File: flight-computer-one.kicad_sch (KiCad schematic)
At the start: 6 parts, among them J1 LEFT_BANK, J2 RIGHT_BANK

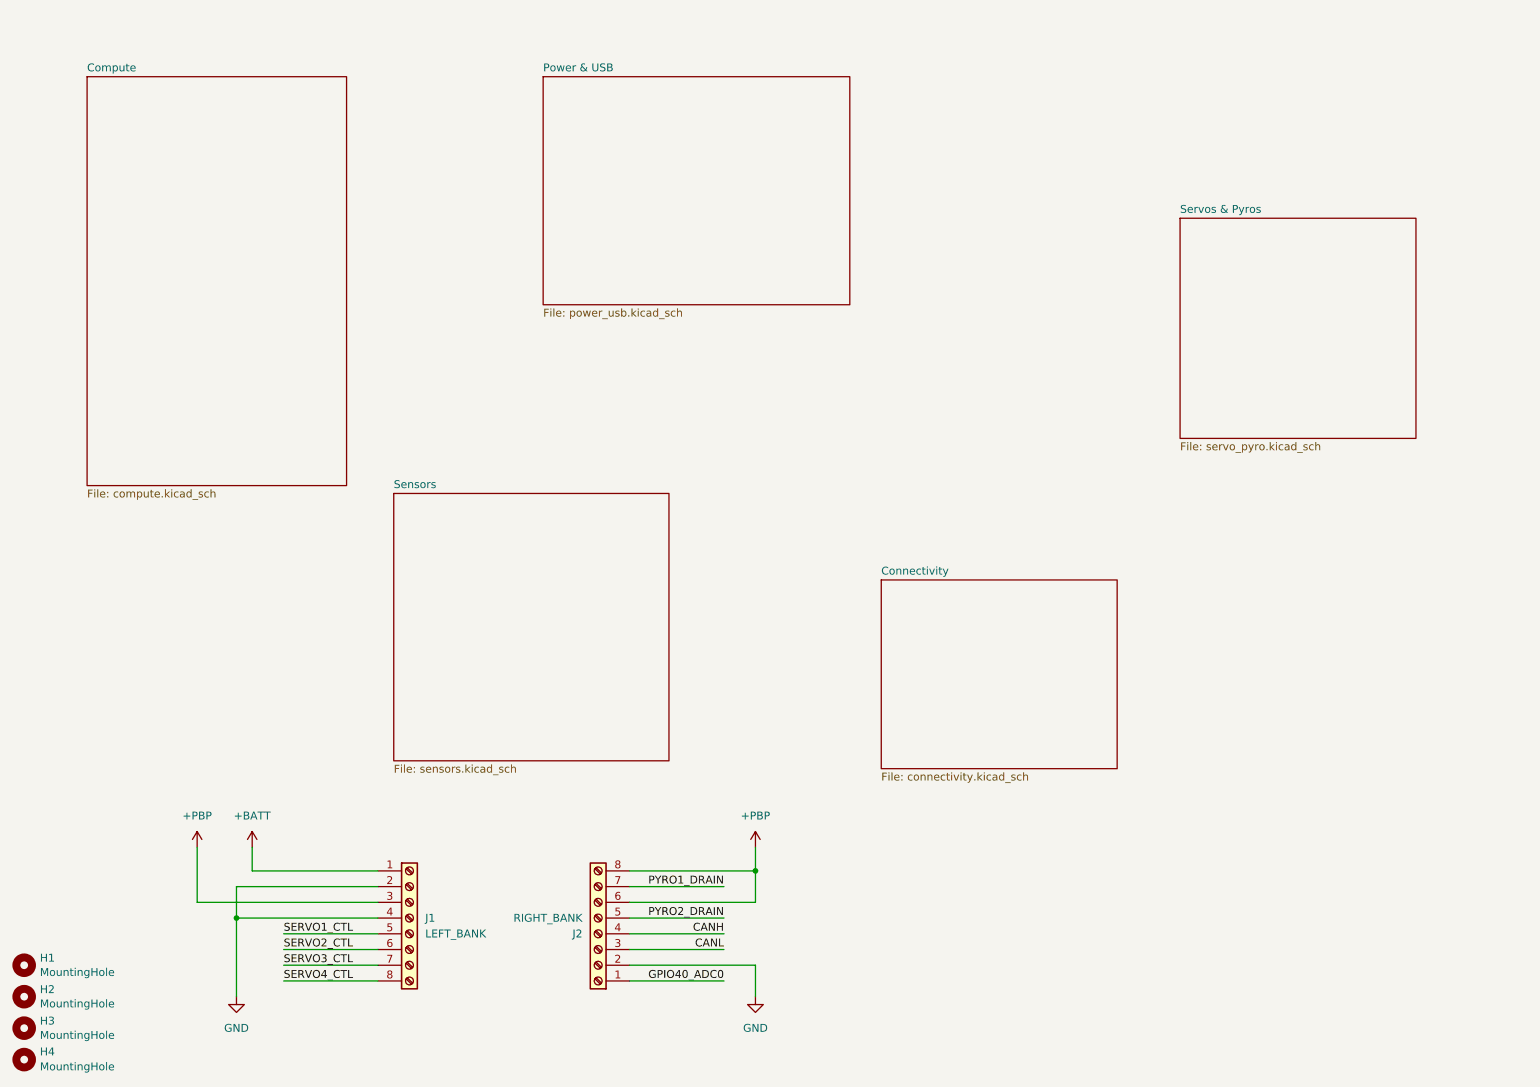
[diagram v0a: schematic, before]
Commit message: schematic tentatively finished
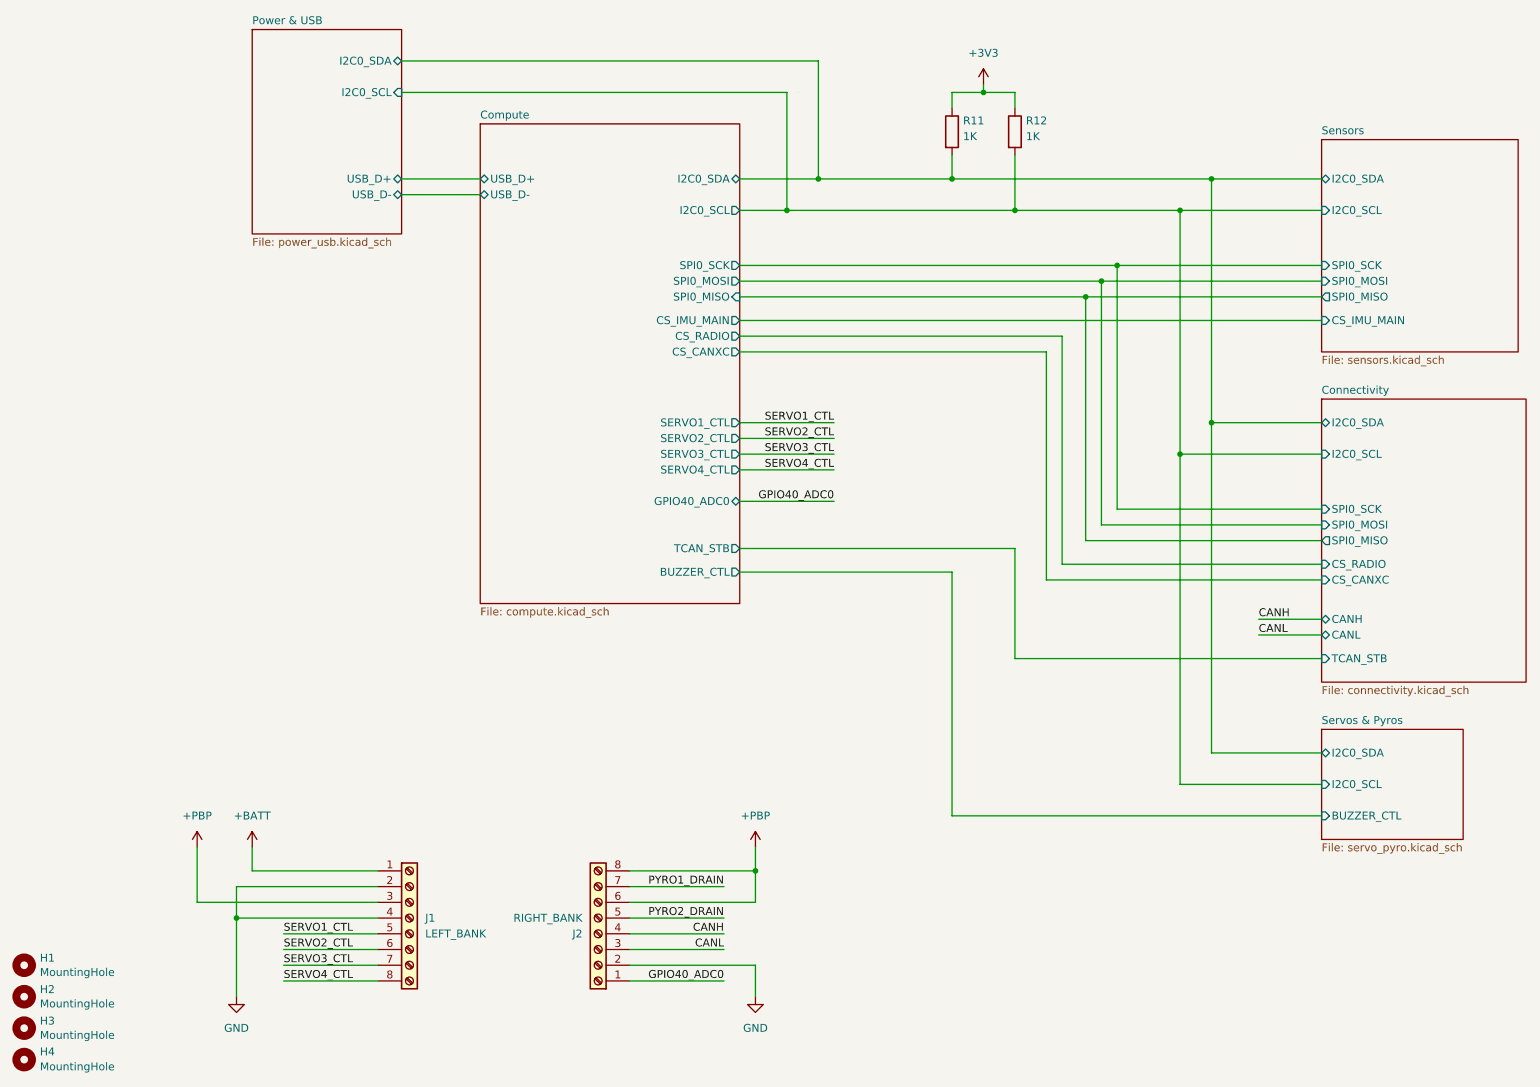
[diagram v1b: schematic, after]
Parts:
- added R11, R12: 1K, Resistor_SMD:R_0603_1608Metric, symbol Device:R
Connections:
- new net +3V3: R11.1, R12.1
- new net Compute/I2C0_SCL: R12.2
- new net Compute/I2C0_SDA: R11.2
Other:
- sheet Compute ports: added BUZZER_CTL, CS_CANXC, CS_IMU_MAIN, CS_RADIO, GPIO40_ADC0, I2C0_SCL, I2C0_SDA, SERVO1_CTL, SERVO2_CTL, SERVO3_CTL, SERVO4_CTL, SPI0_MISO, SPI0_MOSI, SPI0_SCK, TCAN_STB, USB_D+, USB_D-; removed none
- sheet Connectivity ports: added CANH, CANL, CS_CANXC, CS_RADIO, I2C0_SCL, I2C0_SDA, SPI0_MISO, SPI0_MOSI, SPI0_SCK, TCAN_STB; removed none
- sheet Power & USB ports: added I2C0_SCL, I2C0_SDA, USB_D+, USB_D-; removed none
- sheet Sensors ports: added CS_IMU_MAIN, I2C0_SCL, I2C0_SDA, SPI0_MISO, SPI0_MOSI, SPI0_SCK; removed none
- sheet Servos & Pyros ports: added BUZZER_CTL, I2C0_SCL, I2C0_SDA; removed none

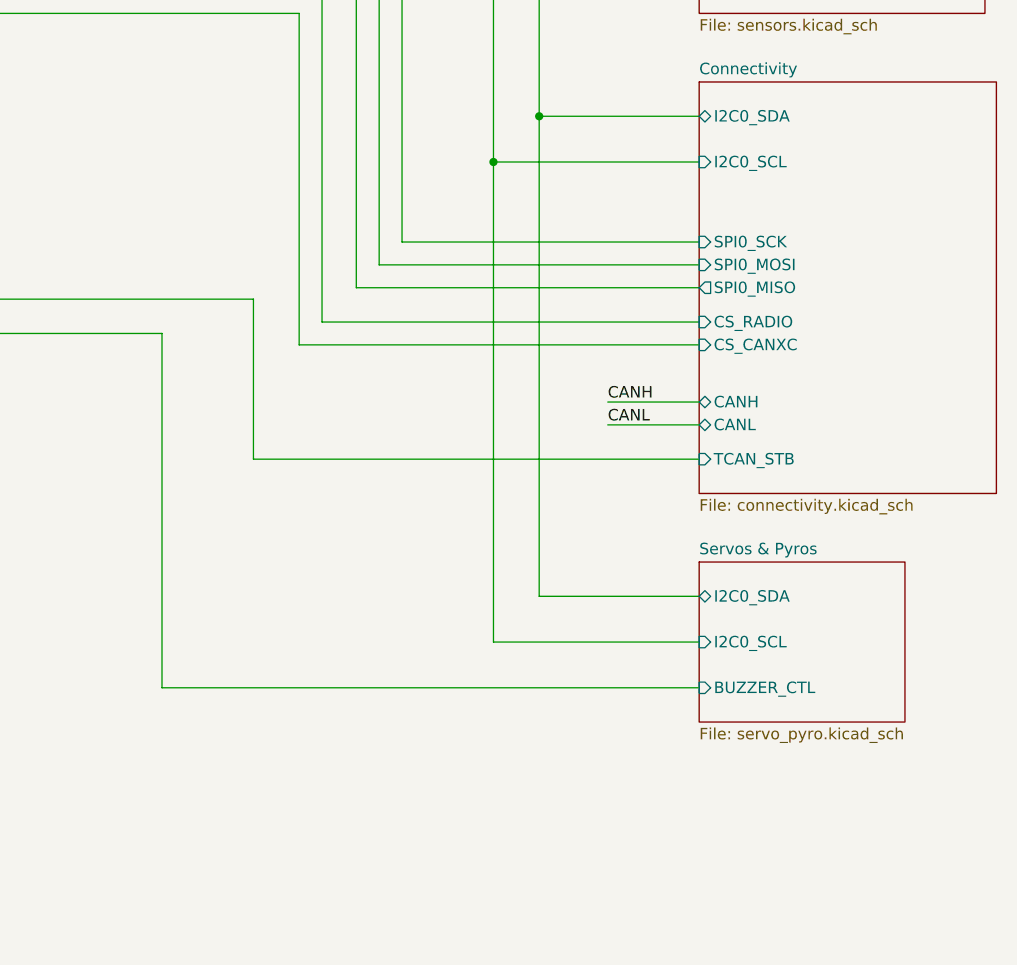
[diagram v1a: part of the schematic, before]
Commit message: preliminary change to SAME51
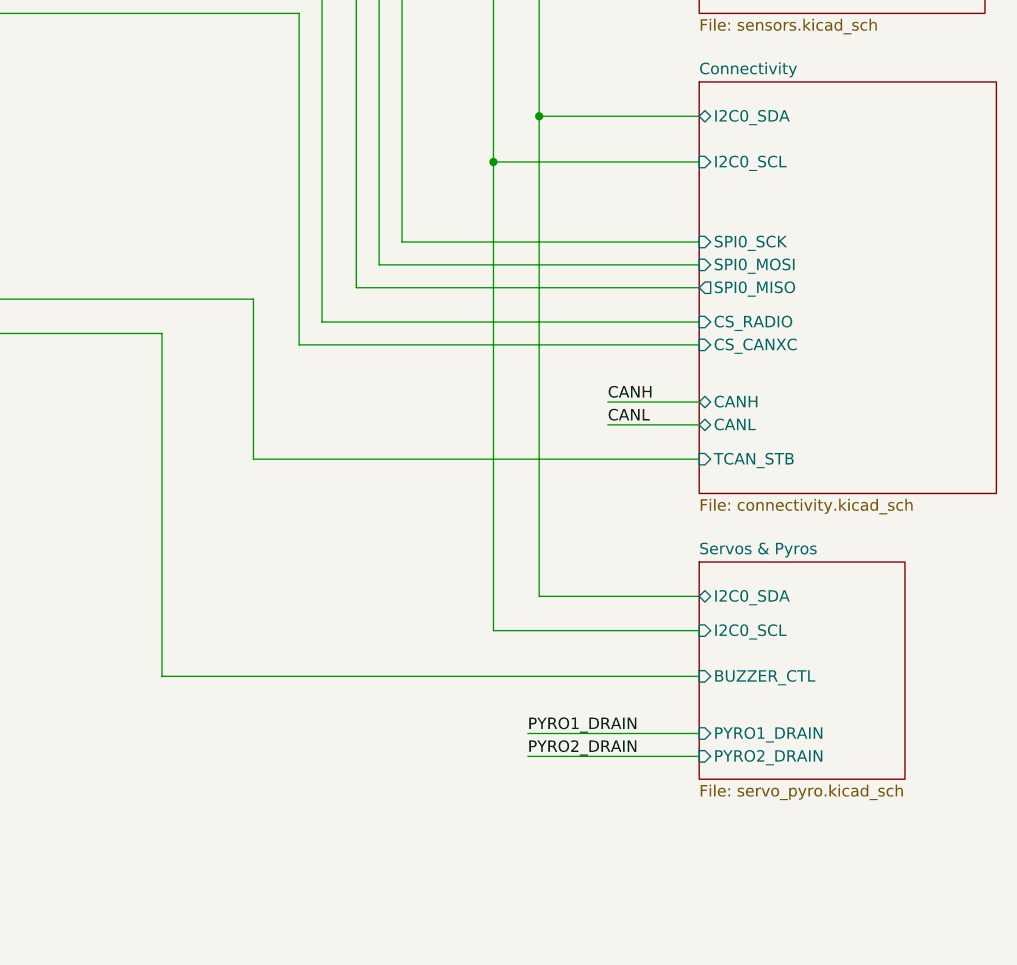
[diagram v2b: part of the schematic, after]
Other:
- sheet Servos & Pyros ports: added PYRO1_DRAIN, PYRO2_DRAIN; removed none
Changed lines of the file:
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@@
 	(wire
 		(pts
-			(xy 173.99 149.86) (xy 233.68 149.86)
+			(xy 173.99 148.59) (xy 233.68 148.59)
 		)
 		(stroke
@@
 	(wire
 		(pts
+			(xy 121.92 166.37) (xy 137.16 166.37)
+		)
+		(stroke
+			(width 0)
+			(type default)
+		)
+	)
+	(wire
+		(pts
 			(xy 184.15 43.18) (xy 184.15 52.07)
 		)
@@
 	(wire
 		(pts
+			(xy 214.63 157.48) (xy 233.68 157.48)
+		)
+		(stroke
+			(width 0)
+			(type default)
+		)
+	)
+	(wire
+		(pts
+			(xy 214.63 154.94) (xy 233.68 154.94)
+		)
+		(stroke
+			(width 0)
+			(type default)
+		)
+	)
+	(wire
+		(pts
 			(xy 223.52 118.11) (xy 233.68 118.11)
 		)
@@
 	(wire
 		(pts
-			(xy 210.82 91.44) (xy 210.82 144.78)
+			(xy 210.82 91.44) (xy 210.82 143.51)
 		)
 		(stroke
@@
 	(wire
 		(pts
-			(xy 121.92 166.37) (xy 137.16 166.37)
-		)
-		(stroke
-			(width 0)
-			(type default)
-		)
-	)
-	(wire
-		(pts
 			(xy 139.7 93.98) (xy 154.94 93.98)
 		)
@@
 	(wire
 		(pts
+			(xy 121.92 161.29) (xy 137.16 161.29)
+		)
+		(stroke
+			(width 0)
+			(type default)
+		)
+	)
+	(wire
+		(pts
 			(xy 85.09 49.53) (xy 97.79 49.53)
 		)
@@
 	(wire
 		(pts
-			(xy 121.92 161.29) (xy 137.16 161.29)
-		)
-		(stroke
-			(width 0)
-			(type default)
-		)
-	)
-	(wire
-		(pts
 			(xy 179.07 31.75) (xy 179.07 33.02)
 		)
@@
 	(wire
 		(pts
-			(xy 210.82 144.78) (xy 233.68 144.78)
+			(xy 210.82 143.51) (xy 233.68 143.51)
 		)
 		(stroke
@@
 	(wire
 		(pts
-			(xy 173.99 110.49) (xy 173.99 149.86)
+			(xy 173.99 110.49) (xy 173.99 148.59)
 		)
 		(stroke
@@
 			(width 0)
 			(type default)
+		)
+	)
+	(label "CANL"
+		(at 137.16 171.45 180)
+		(effects
+			(font
+				(size 1.27 1.27)
+			)
+			(justify right bottom)
+		)
+	)
+	(label "SERVO1_CTL"
+		(at 154.94 86.36 180)
+		(effects
+			(font
+				(size 1.27 1.27)
+			)
+			(justify right bottom)
+		)
+	)
+	(label "SERVO2_CTL"
+		(at 66.04 171.45 0)
+		(effects
+			(font
+				(size 1.27 1.27)
+			)
+			(justify left bottom)
+		)
+	)
+	(label "SERVO4_CTL"
+		(at 66.04 176.53 0)
+		(effects
+			(font
+				(size 1.27 1.27)
+			)
+			(justify left bottom)
+		)
+	)
+	(label "CANH"
+		(at 137.16 168.91 180)
+		(effects
+			(font
+				(size 1.27 1.27)
+			)
+			(justify right bottom)
+		)
+	)
+	(label "PYRO2_DRAIN"
+		(at 214.63 157.48 0)
+		(effects
+			(font
+				(size 1.27 1.27)
+			)
+			(justify left bottom)
+		)
+	)
+	(label "GPIO40_ADC0"
+		(at 154.94 99.06 180)
+		(effects
+			(font
+				(size 1.27 1.27)
+			)
+			(justify right bottom)
 		)
 	)
@@
 		)
 	)
-	(label "CANL"
-		(at 137.16 171.45 180)
+	(label "CANH"
+		(at 223.52 118.11 0)
 		(effects
 			(font
 				(size 1.27 1.27)
 			)
-			(justify right bottom)
-		)
-	)
-	(label "SERVO1_CTL"
-		(at 154.94 86.36 180)
+			(justify left bottom)
+		)
+	)
+	(label "GPIO40_ADC0"
+		(at 137.16 176.53 180)
 		(effects
 			(font
@@
 		)
 	)
-	(label "SERVO2_CTL"
-		(at 66.04 171.45 0)
-		(effects
-			(font
-				(size 1.27 1.27)
-			)
-			(justify left bottom)
-		)
-	)
-	(label "SERVO4_CTL"
-		(at 66.04 176.53 0)
+	(label "CANL"
+		(at 223.52 120.65 0)
 		(effects
 			(font
@@
 		)
 	)
-	(label "CANH"
-		(at 137.16 168.91 180)
-		(effects
-			(font
-				(size 1.27 1.27)
-			)
-			(justify right bottom)
-		)
-	)
-	(label "GPIO40_ADC0"
-		(at 154.94 99.06 180)
-		(effects
-			(font
-				(size 1.27 1.27)
-			)
-			(justify right bottom)
-		)
-	)
-	(label "CANH"
-		(at 223.52 118.11 0)
-		(effects
-			(font
-				(size 1.27 1.27)
-			)
-			(justify left bottom)
-		)
-	)
-	(label "GPIO40_ADC0"
-		(at 137.16 176.53 180)
-		(effects
-			(font
-				(size 1.27 1.27)
-			)
-			(justify right bottom)
-		)
-	)
-	(label "CANL"
-		(at 223.52 120.65 0)
-		(effects
-			(font
-				(size 1.27 1.27)
-			)
-			(justify left bottom)
-		)
-	)
 	(label "SERVO4_CTL"
 		(at 154.94 93.98 180)
@@
 			)
 			(justify right bottom)
+		)
+	)
+	(label "PYRO1_DRAIN"
+		(at 214.63 154.94 0)
+		(effects
+			(font
+				(size 1.27 1.27)
+			)
+			(justify left bottom)
 		)
 	)
@@
 	(sheet
 		(at 233.68 135.89)
-		(size 22.86 17.78)
+		(size 22.86 24.13)
 		(exclude_from_sim no)
 		(in_bom yes)
@@
 		)
 		(property "Sheetfile" "servo_pyro.kicad_sch"
-			(at 233.68 154.2546 0)
+			(at 233.68 160.6046 0)
 			(effects
 				(font
@@
 		)
 		(pin "BUZZER_CTL" input
-			(at 233.68 149.86 180)
+			(at 233.68 148.59 180)
 			(effects
 				(font
@@
 		)
 		(pin "I2C0_SCL" input
-			(at 233.68 144.78 180)
+			(at 233.68 143.51 180)
 			(effects
 				(font
@@
 			(effects
 				(font
+					(size 1.27 1.27)
+				)
+				(justify left)
+			)
+		)
+		(pin "PYRO1_DRAIN" input
+			(at 233.68 154.94 180)
+			(effects
+				(font
+					(size 1.27 1.27)
+				)
+				(justify left)
+			)
+		)
+		(pin "PYRO2_DRAIN" input
+			(at 233.68 157.48 180)
+			(effects
+				(font
